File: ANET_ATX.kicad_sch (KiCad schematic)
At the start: 13 parts, among them J1 External connect, J2ATX1 39-30-1200, J3USB1 292303-7, J4 39357-0002, J5 39357-0002, J6RPI1 BLG2X20, Q1 2N3904, SW1HWSTART1 SW_DIP_x01

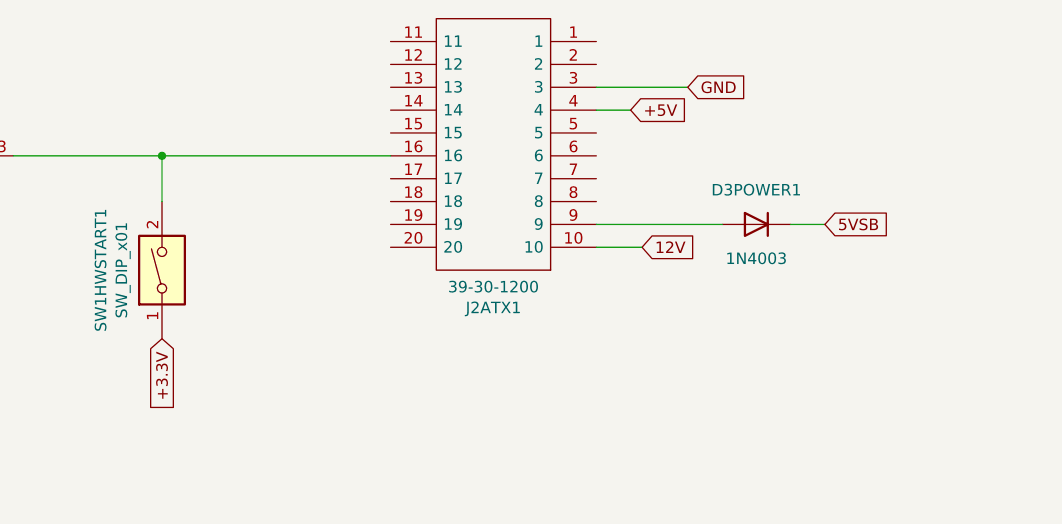
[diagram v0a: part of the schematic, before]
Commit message: replaced best parts
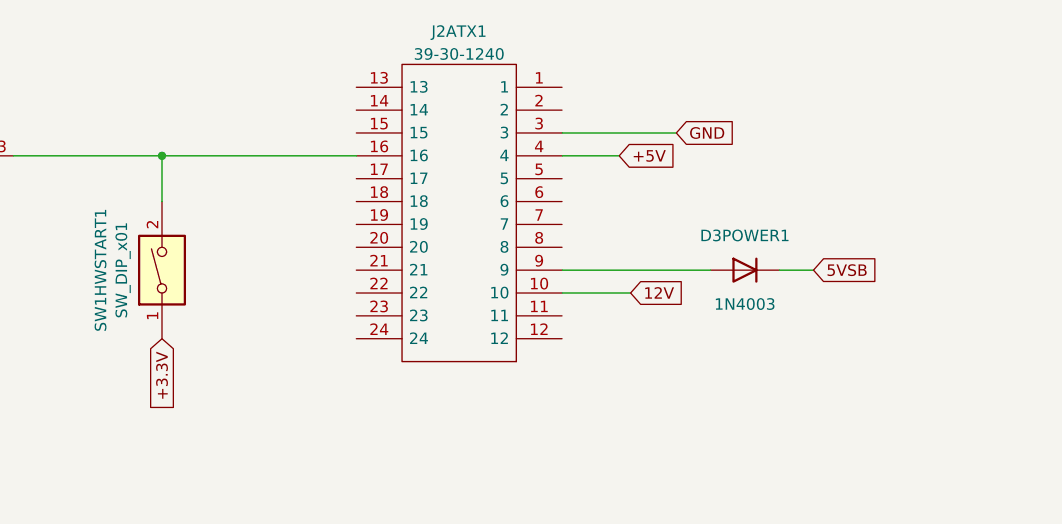
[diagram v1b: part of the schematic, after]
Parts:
- removed J2ATX1: 39-30-1200, SamacSys_Parts:39-30-120Y_012, symbol ANET_ATX-rescue:39-30-1200-SamacSys_Parts
- added J2ATX1: 39-30-1240, SamacSys_Parts:39-30-124Y_012, symbol SamacSys_Parts:39-30-1240
- J3USB1: footprint SamacSys_Parts:2923037 -> SamacSys_Parts:A-USBSA
- J4, J5: footprint SamacSys_Parts:393570002 -> SamacSys_Parts:0398800302
- J6RPI1: footprint SamacSys_Parts:RHDR40W64P254X254_2X20_5130X500X865P -> SamacSys_Parts:RHDR40W64P254_2X20_5130X500X1375P
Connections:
- net +5V: now also J2ATX1.4
- net 12V: now also J2ATX1.10
- net GND: now also J2ATX1.3
- net at Q1.3 (E), SW1HWSTART1.2: now also J2ATX1.16
- net at D3POWER1.2 (A): now also J2ATX1.9
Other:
- moved on the sheet: D3POWER1
